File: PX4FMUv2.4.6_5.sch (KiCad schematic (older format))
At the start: 21 parts, among them U501 L3GD20, U502 L3GD20H, U504 LSM303D, U505 MPU-6000, U506 MS5611-01BA, X503 0512811094

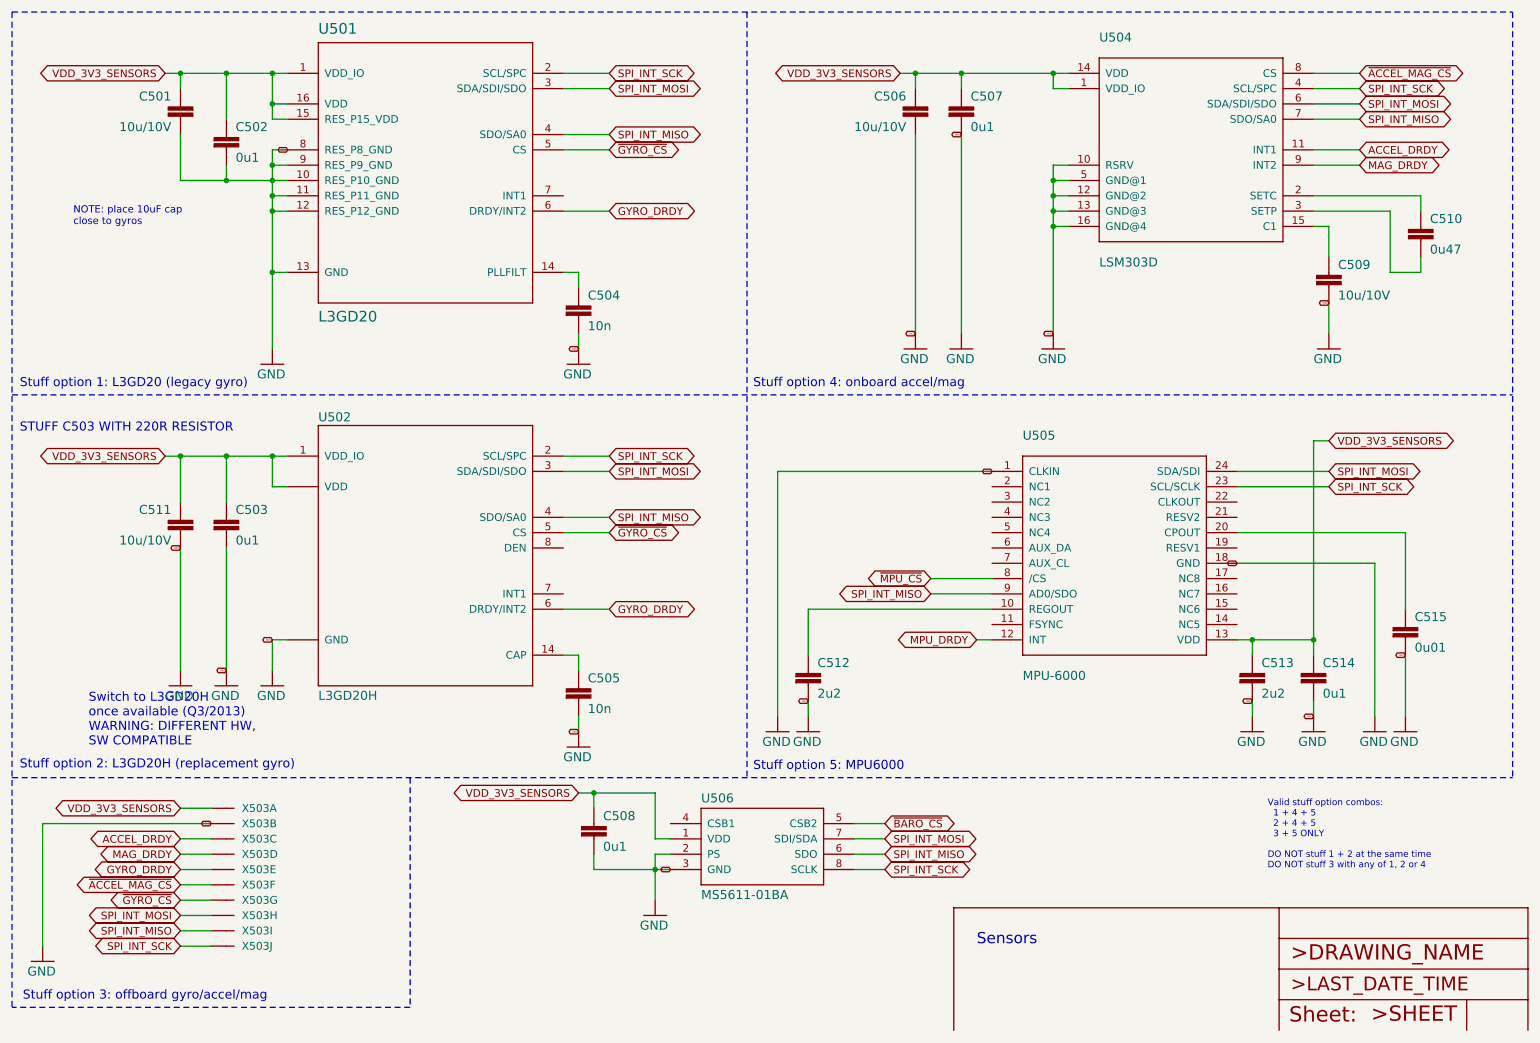
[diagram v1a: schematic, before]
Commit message: removed more things
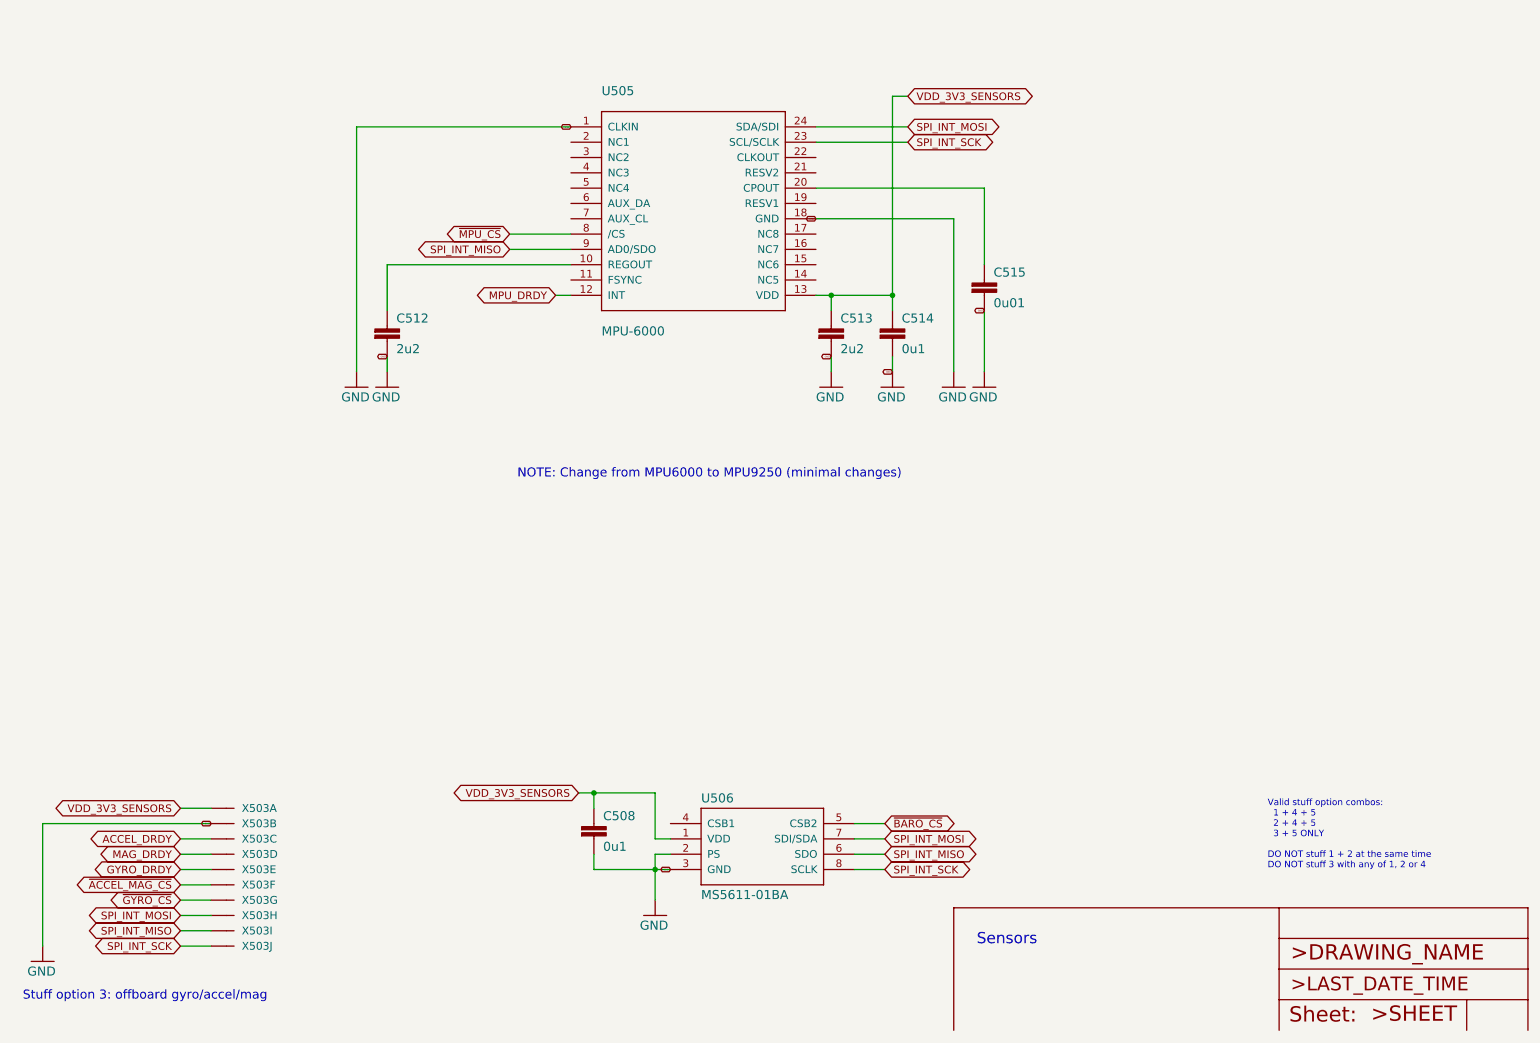
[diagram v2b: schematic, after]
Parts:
- removed C501, C506, C509, C511: 10u/10V, PX4FMUv2.4.6:0805-CAP, symbol PX4FMUv2.4.6-eagle-import:CAP0805
- removed C502, C503, C507: 0u1, PX4FMUv2.4.6:0402-CAP, symbol PX4FMUv2.4.6-eagle-import:CAP0402
- removed C504, C505: 10n, PX4FMUv2.4.6:0402-CAP, symbol PX4FMUv2.4.6-eagle-import:CAP0402
- removed C510: 0u47, PX4FMUv2.4.6:0402-CAP, symbol PX4FMUv2.4.6-eagle-import:CAP0402
- removed U501: L3GD20, PX4FMUv2.4.6:L3G4200DH-MAN, symbol PX4FMUv2.4.6-eagle-import:L3G4200DH-LL
- removed U502: L3GD20H, PX4FMUv2.4.6:LGA-16L, symbol PX4FMUv2.4.6-eagle-import:L3GD20H
- removed U504: LSM303D, PX4FMUv2.4.6:LGA-16L, symbol PX4FMUv2.4.6-eagle-import:LSM303D
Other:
- note added: "NOTE: Change from MPU6000 to MPU9250 (minimal changes)"
- note removed: "NOTE: place 10uF cap\nclose to gyros"
- note removed: "STUFF C503 WITH 220R RESISTOR"
- note removed: "Stuff option 1: L3GD20 (legacy gyro)"
- note removed: "Stuff option 2: L3GD20H (replacement gyro)"
- note removed: "Stuff option 4: onboard accel/mag"
- note removed: "Stuff option 5: MPU6000"
- note removed: "Switch to L3GD20H\nonce available (Q3/2013)\nWARNING: DIFFERENT HW,\nSW COMPATIBLE"
- moved on the sheet: C512, C513, C514, C515, U505
